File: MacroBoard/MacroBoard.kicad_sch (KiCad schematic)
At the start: 80 parts, among them J1 USB_C_Receptacle_USB2.0, SW1 SW_Push, U1 AT90USB1286-AU, Y1 Crystal_GND24_Small

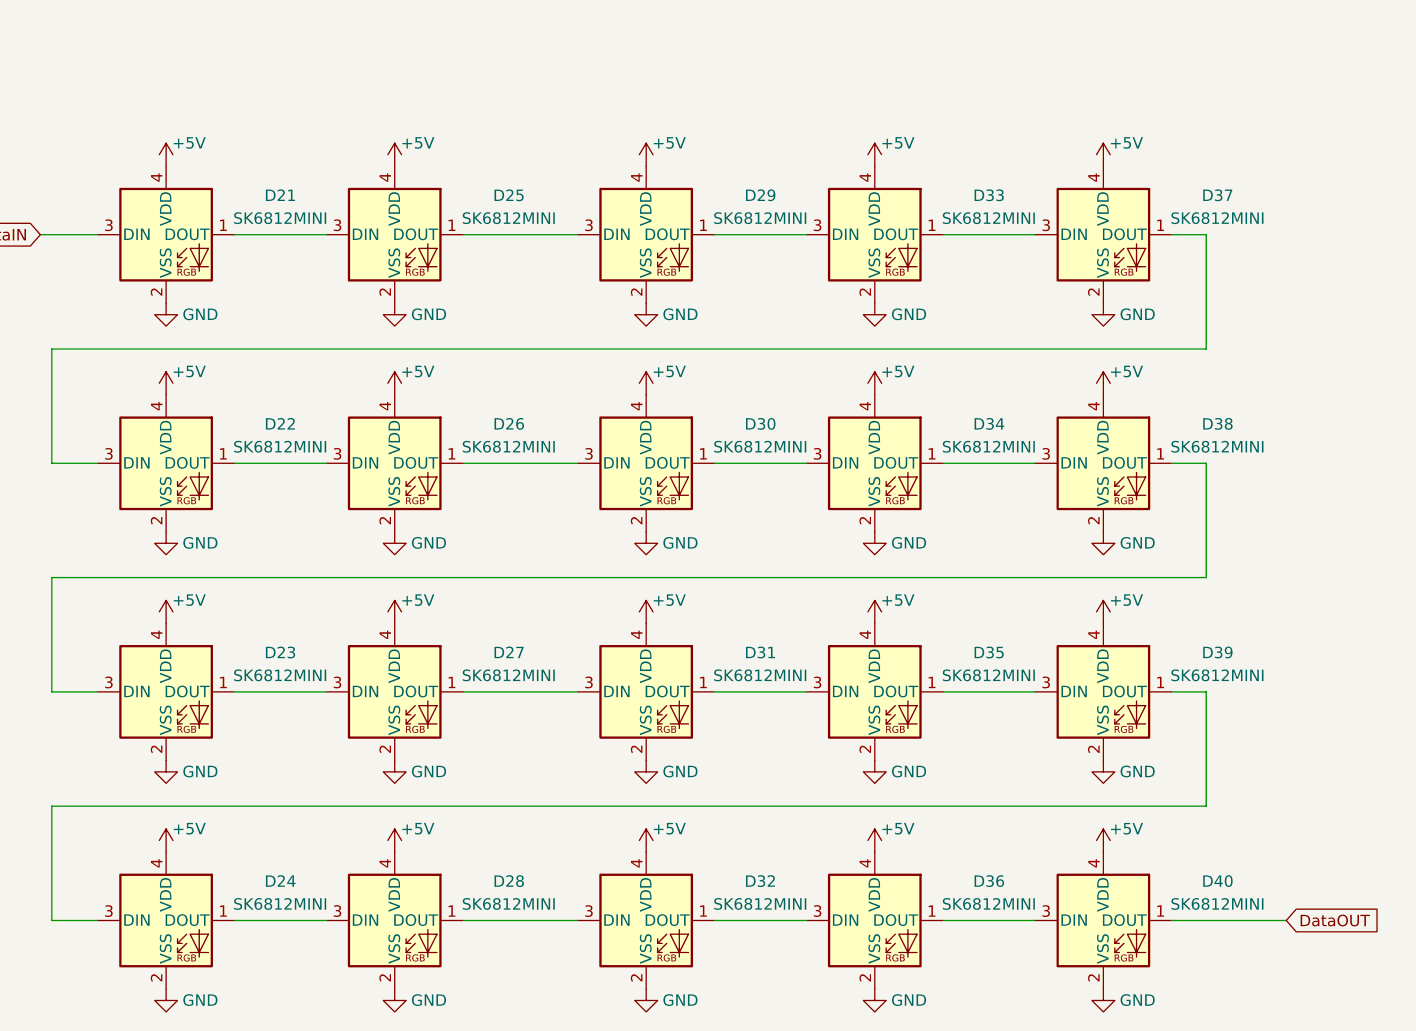
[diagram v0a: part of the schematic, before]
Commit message: macro board
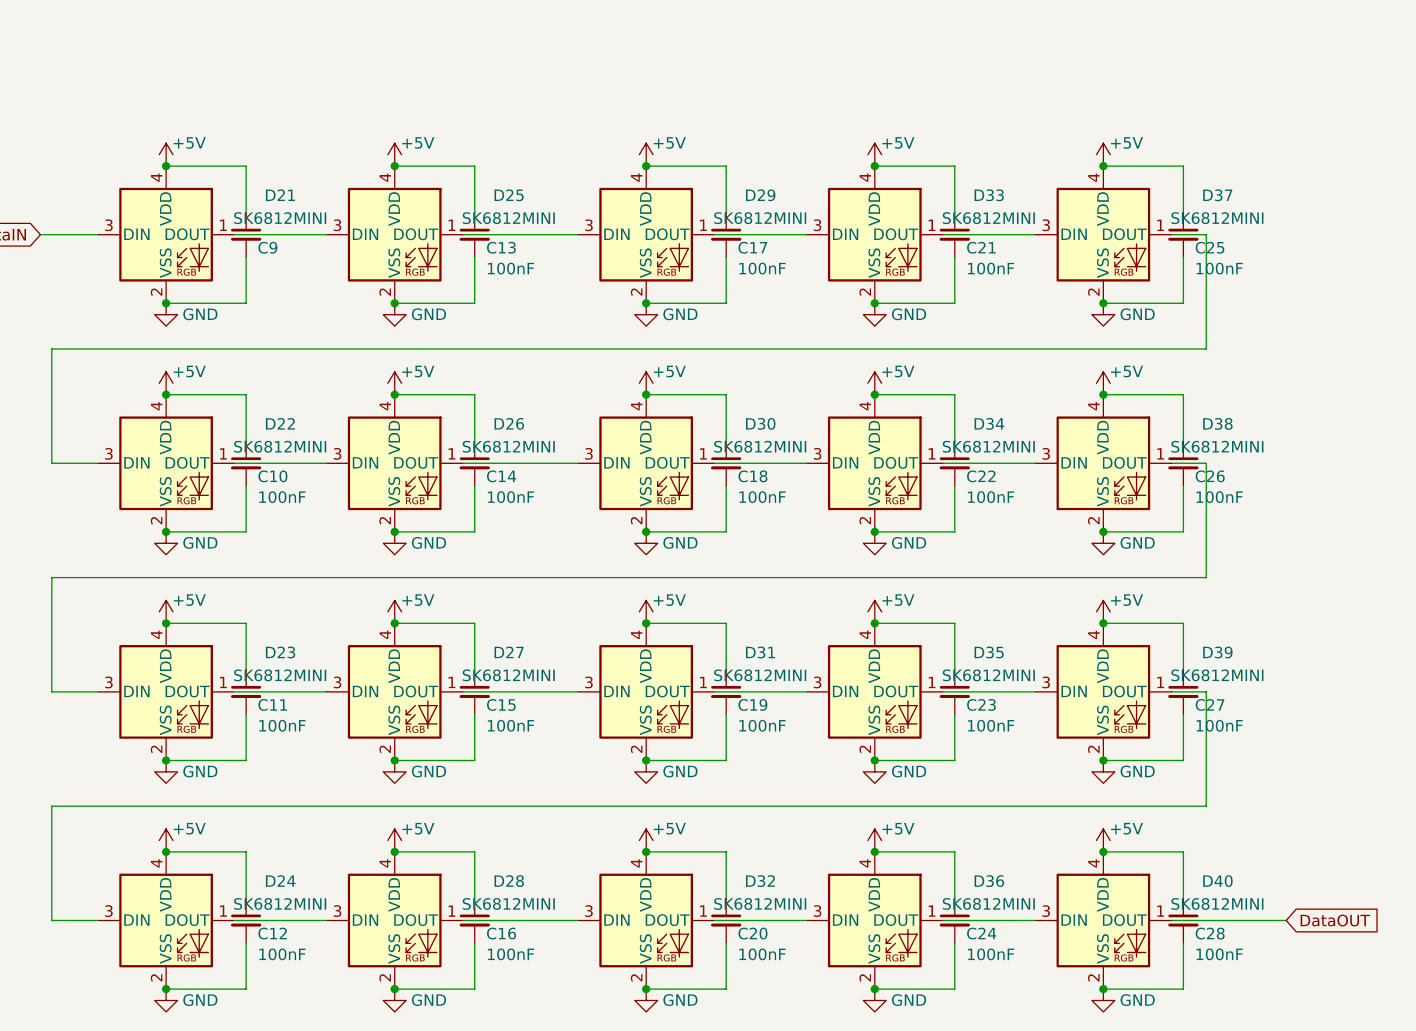
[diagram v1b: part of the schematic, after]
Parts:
- added C10, C11, C12, C13, C14, C15, C16, C17, C18, C19, C20, C21, C22, C23, C24, C25, C26, C27, C28: 100nF, symbol Device:C_Small
- added C9: (no value), symbol Device:C_Small
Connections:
- net +5V: now also C10.1, C11.1, C12.1, C13.1, C14.1, C15.1, C16.1, C17.1, C18.1, C19.1, C20.1, C21.1, C22.1, C23.1, C24.1, C25.1, C26.1, C27.1, C28.1, C9.1
- net GND: now also C10.2, C11.2, C12.2, C13.2, C14.2, C15.2, C16.2, C17.2, C18.2, C19.2, C20.2, C21.2, C22.2, C23.2, C24.2, C25.2, C26.2, C27.2, C28.2, C9.2

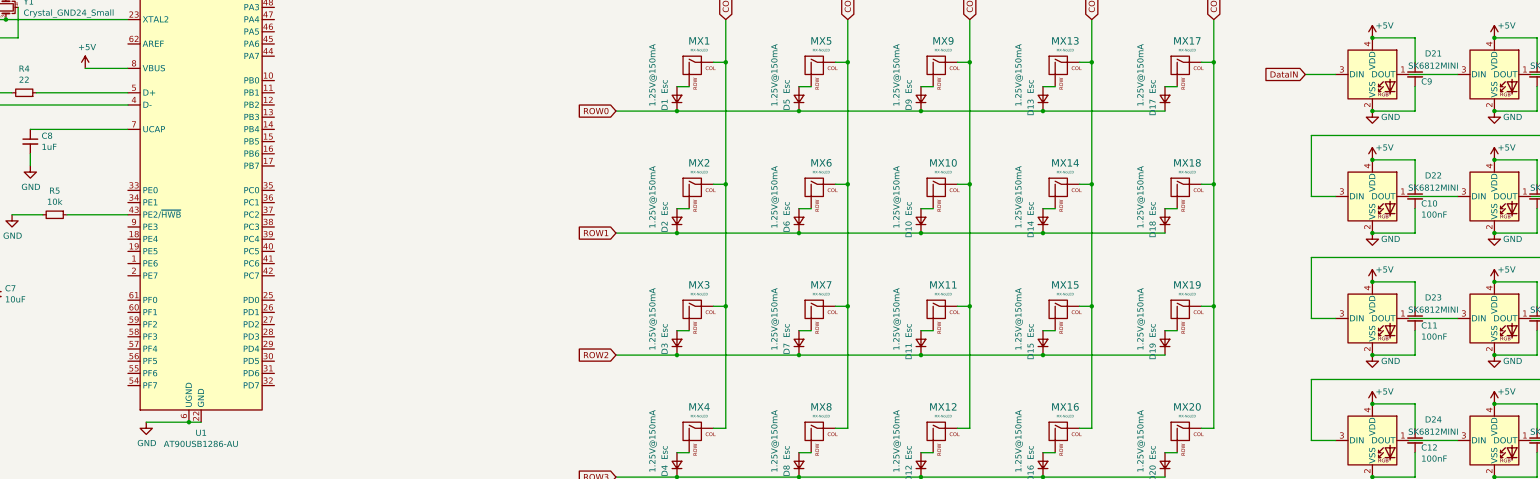
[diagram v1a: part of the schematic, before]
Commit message: makro board
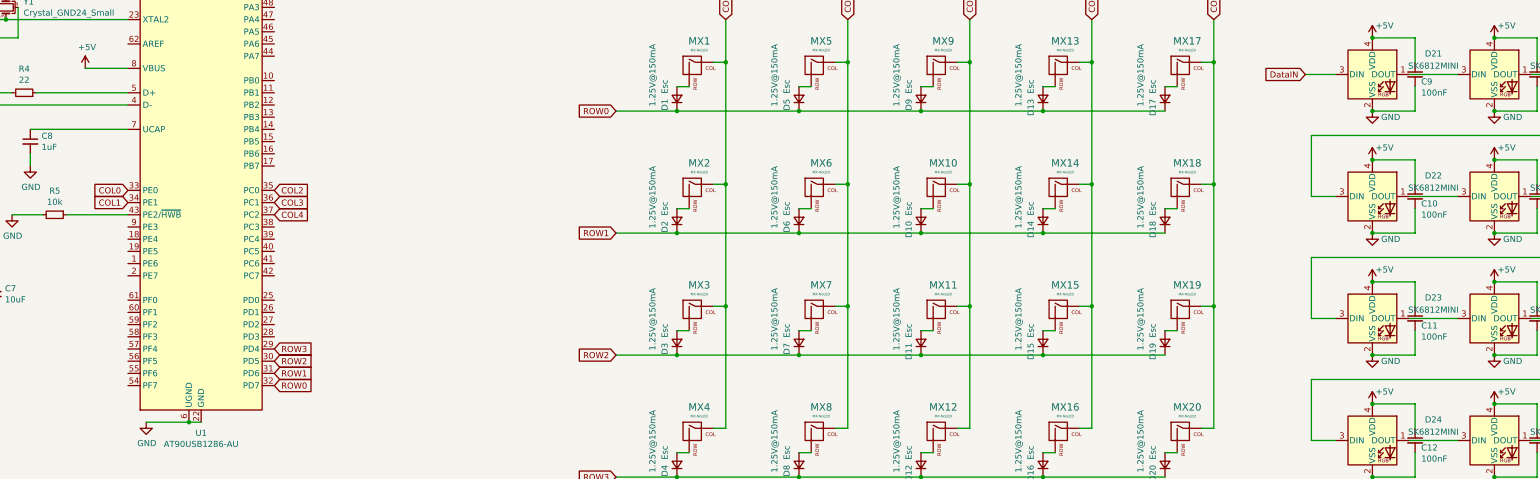
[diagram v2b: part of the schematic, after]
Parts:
- C10, C11, C12, C13, C14, C15, C16, C17, C18, C19, C20, C21, C22, C23, C24, C25, C26, C27, C28: footprint (none) -> led:led_capacitor
- C9: value (none) -> 100nF; footprint (none) -> led:led_capacitor
- D21, D22, D23, D24, D25, D26, D27, D28, D29, D30, D31, D32, D33, D34, D35, D36, D37, D38, D39, D40: footprint (none) -> led:SK6812MINI_3.5x3.7mm_SMD-Flipped-Back
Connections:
- net COL0: now also U1.33 (PE0)
- net COL1: now also U1.34 (PE1)
- net COL2: now also U1.35 (PC0)
- net COL3: now also U1.36 (PC1)
- net COL4: now also U1.37 (PC2)
- net ROW0: now also U1.32 (PD7)
- net ROW1: now also U1.31 (PD6)
- net ROW2: now also U1.30 (PD5)
- net ROW3: now also U1.29 (PD4)
